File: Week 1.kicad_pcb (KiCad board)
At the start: 2 copper layers, 96.5 x 50 mm, 7 parts, among them J1 Conn_01x04_Pin, J2 Conn_01x08_Pin, SW1 SW_Push, SW2 SW_Push, U1 XIAO-ESP32-C3-SMD, U2 DHT11

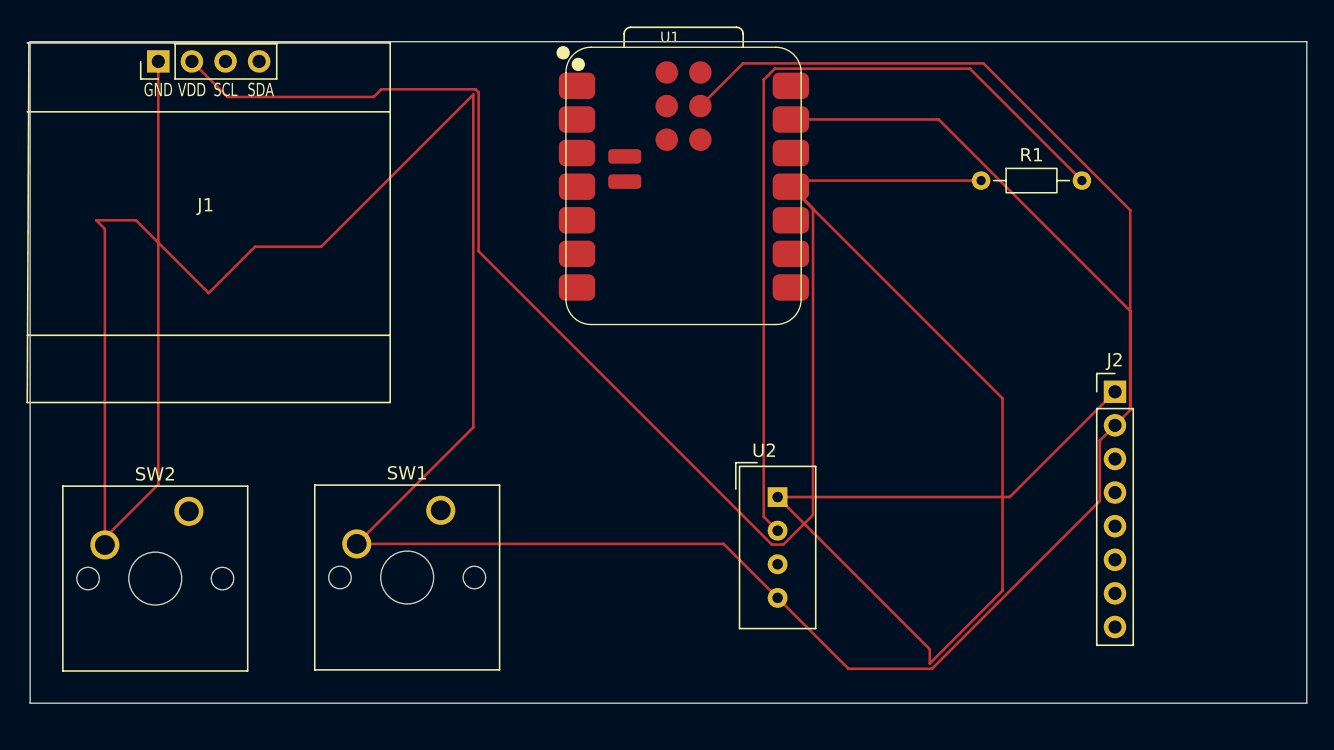
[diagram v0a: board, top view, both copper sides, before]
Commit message: added many things
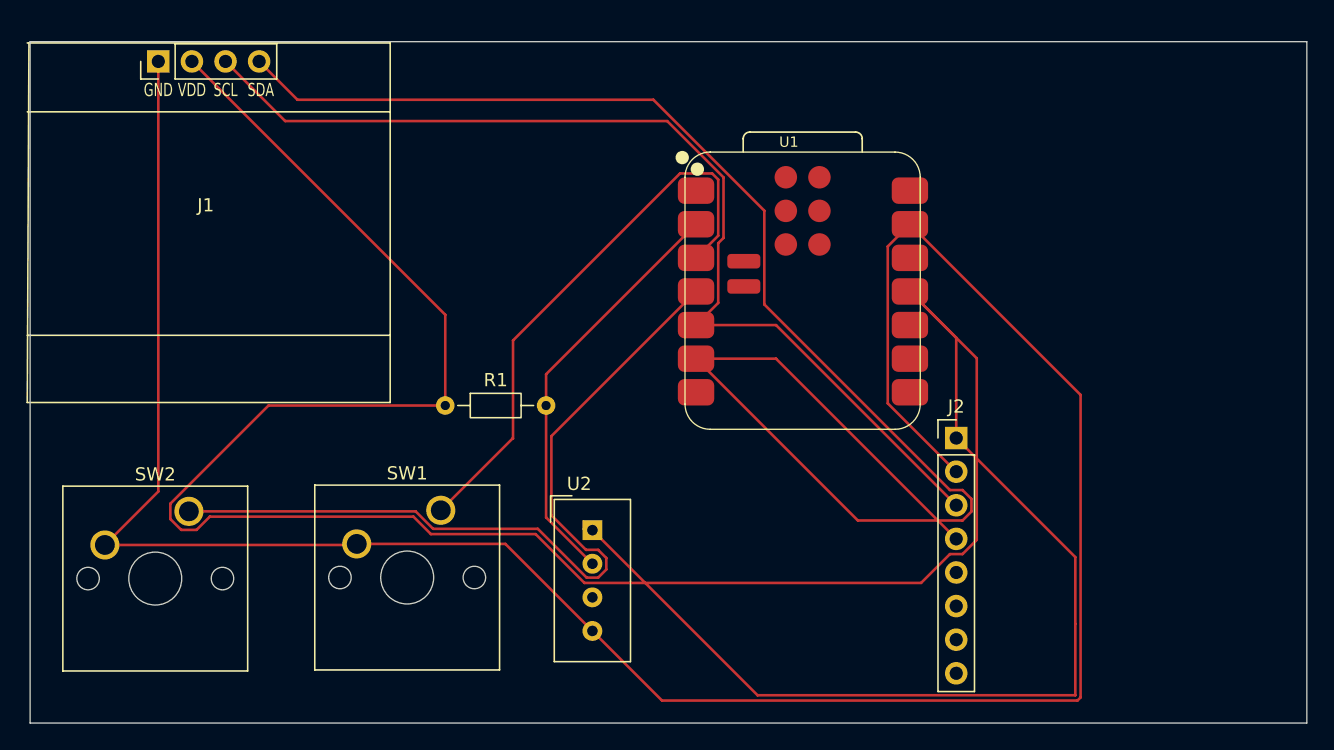
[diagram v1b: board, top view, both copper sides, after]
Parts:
- moved R1 43.9 mm to (141.4, 92.5)
- moved U2 14.2 mm to (152.5, 101.9)
- moved J2 12.5 mm to (180.0, 95.0)
- moved U1 12.0 mm to (159.5, 94.4)
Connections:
- J1 pad 3: unconnected-(J1-Pin_3-Pad3) -> /SCL
- J1 pad 4: unconnected-(J1-Pin_4-Pad4) -> /SDA
- J2 pad 3: unconnected-(J2-Pin_3-Pad3) -> /SCL
- J2 pad 4: unconnected-(J2-Pin_4-Pad4) -> /SDA
- U1 pad 2: unconnected-(U1-D1-Pad2) -> /DHT11 DATA
- U1 pad 3: unconnected-(U1-D2-Pad3) -> /GPIO 2
- U1 pad 4: unconnected-(U1-D3-Pad4) -> /GPIO 3
- U1 pad 5: unconnected-(U1-D4-Pad5) -> /SCL
- U1 pad 6: unconnected-(U1-D5-Pad6) -> /SDA
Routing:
- net /SDA: track 0.00 -> 124.3 mm
- net GND: track 303.5 -> 180.2 mm
- net /SCL: track 0.00 -> 78.6 mm
- net /GPIO 3: track 0.00 -> 61.7 mm
- net /GPIO 2: track 0.00 -> 42.7 mm
- net /DHT11 DATA: track 62.4 -> 31.8 mm
- net +3.3V: track 201.7 -> 223.8 mm
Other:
- board size 96.5 x 50 mm -> 96.5 x 51.5 mm
